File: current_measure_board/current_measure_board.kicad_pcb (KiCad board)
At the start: 6 copper layers, 76.2 x 76.2 mm, 43 parts, among them U1 LT6370HMS8-TRPBF, U2 LT1793AIS8-PBF, U3 LT1793AIS8-PBF, U4 LT1793AIS8-PBF

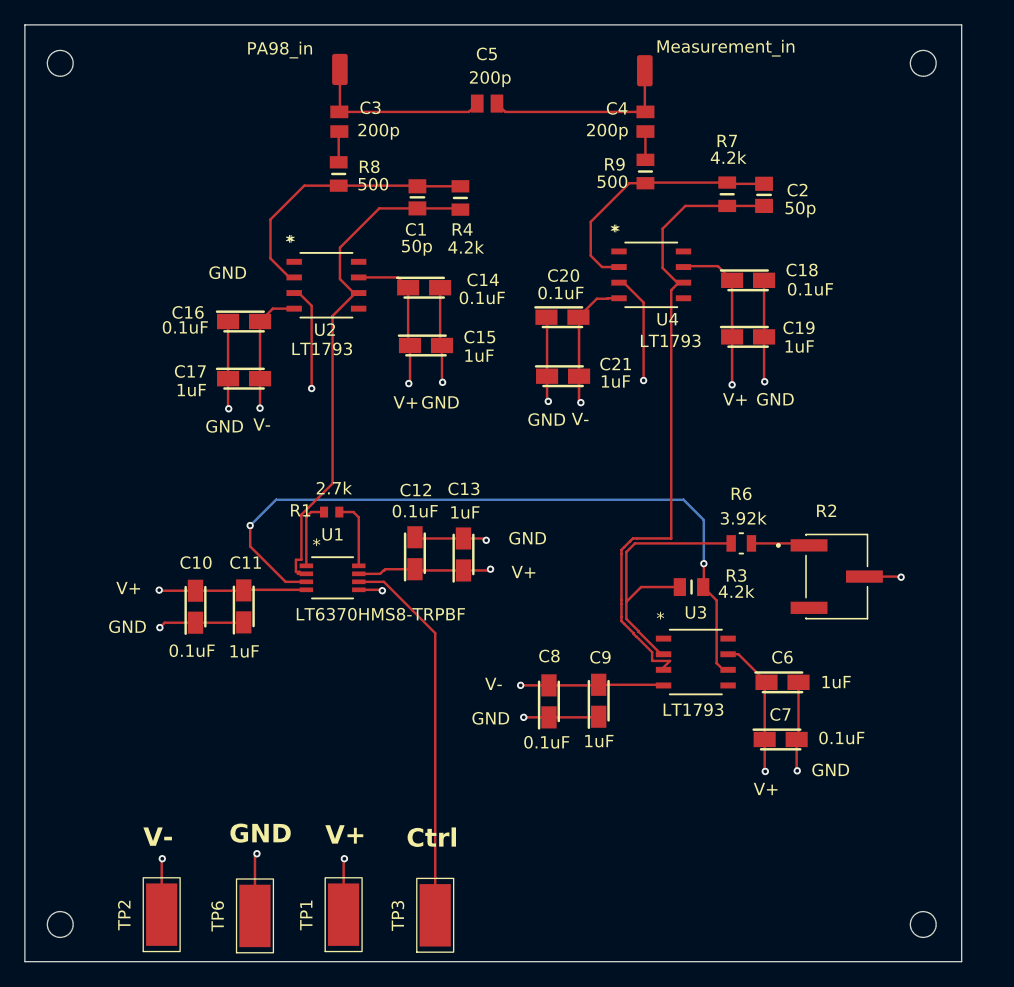
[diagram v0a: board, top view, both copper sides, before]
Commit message: current board update
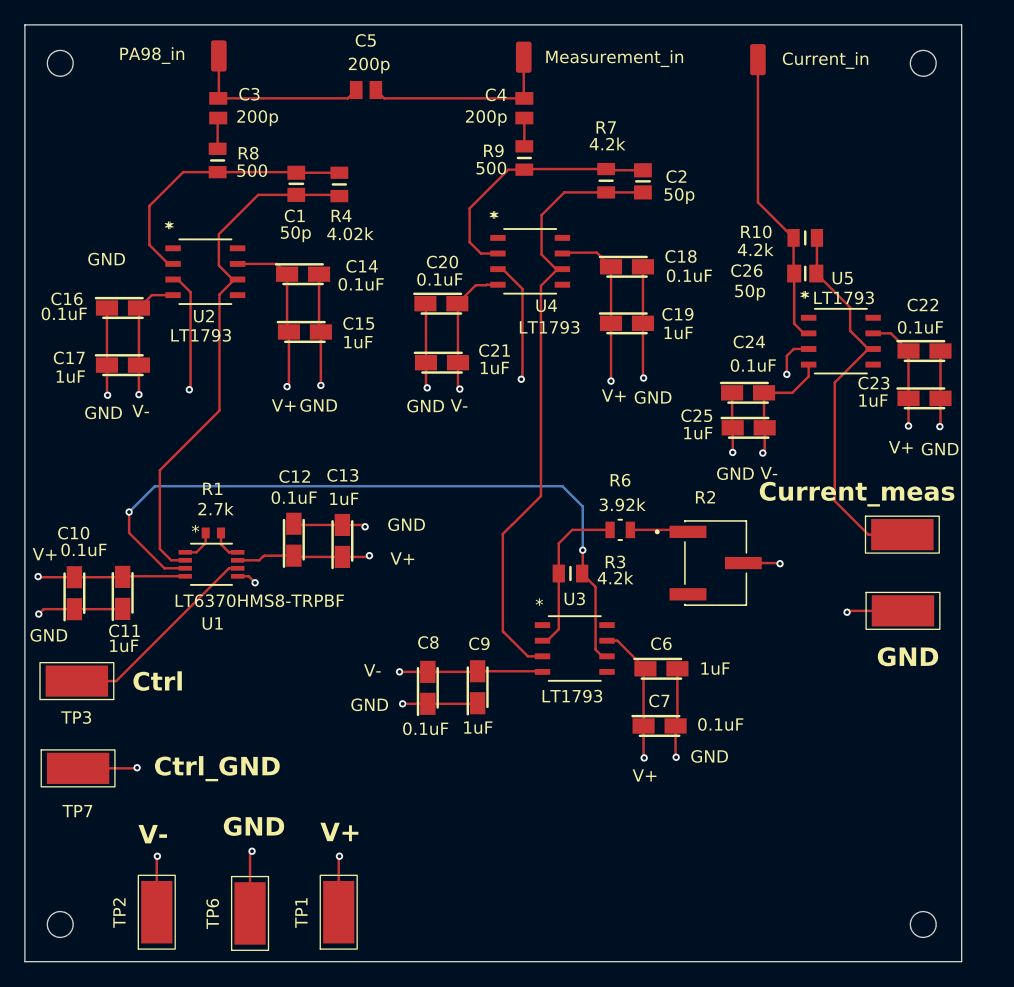
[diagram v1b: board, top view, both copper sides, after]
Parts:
- added C22: C1206C104K5RACTM, Custom_capacitors:CAPPM3216X180N(0.1uF 1206 0.1acc), F.Cu at (182.7, 84.2)
- added C23: TH3A105K035D6600, Custom_capacitors:CAPPM3216X180N(1uF 35V 1206 0.1err, F.Cu at (182.7, 88.1)
- added C24: C1206C104K5RACTM, Custom_capacitors:CAPPM3216X180N(0.1uF 1206 0.1acc), F.Cu at (168.3, 87.7)
- added C25: TH3A105K035D6600, Custom_capacitors:CAPPM3216X180N(1uF 35V 1206 0.1err, F.Cu at (168.4, 90.5)
- added C26: 50p, Custom_capacitors:CAPC2012X140N(50pF 1206 1 C0G 100V), F.Cu at (173.0, 78.0)
- added R10: 4.2k, Custom_resistors:RESC2012X55N(4.02k Ohm 0805 0.1err), F.Cu at (173.0, 75.0)
- added TP10: TestPoint, Custom_testpoint:PAD_EXT_0.635x2.54mm, F.Cu at (169.2, 60.5)
- added TP7: TestPoint, Custom_trimpot:PAD_EXT_2.54x5.08mm, F.Cu at (113.8, 120.7)
- added TP8: TestPoint, Custom_trimpot:PAD_EXT_2.54x5.08mm, F.Cu at (180.9, 101.7)
- added TP9: TestPoint, Custom_trimpot:PAD_EXT_2.54x5.08mm, F.Cu at (180.9, 107.9)
- added U5: LT1793AIS8-PBF, Custom_amplifiers:LT1793AIS_8_PBF, F.Cu at (175.9, 83.5)
- moved TP3 38.3 mm to (113.8, 108.6), turned to 180 degrees
- moved C21 9.91 mm to (143.4, 85.2)
- moved R6 9.91 mm to (157.9, 98.8)
- moved U4 9.91 mm to (150.6, 77.0)
- moved C10 9.91 mm to (113.5, 104.0)
- moved C11 9.91 mm to (117.5, 103.9)
- moved R8 9.91 mm to (125.2, 68.8)
- moved TP4 9.91 mm to (125.3, 60.2)
- moved U1 9.91 mm to (124.7, 101.6)
- moved U2 9.91 mm to (124.2, 77.8)
- moved C1 9.91 mm to (131.6, 70.7)
- moved C12 9.91 mm to (131.4, 99.6)
- moved C13 9.91 mm to (135.3, 99.7)
- moved C14 9.91 mm to (132.2, 78.0)
- moved C15 9.91 mm to (132.3, 82.7)
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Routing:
- net /Current_meas: track 0.00 -> 31.3 mm
- net GND: track 84.1 -> 112.2 mm, vias 13 -> 18
- net /Current_in: track 0.00 -> 24.2 mm
- net /Control_out: track 30.9 -> 16.9 mm
- net /Vplus: track 52.5 -> 64.3 mm, vias 5 -> 6
- net /Vminus: track 49.8 -> 59.9 mm, vias 5 -> 6
- net Net-(U3--INA): track 23.4 -> 13.5 mm
- net Net-(U1-RG+): track 5.70 -> 2.55 mm
- net Net-(U1-RG-): track 5.59 -> 2.80 mm
- net Net-(U3-+INA): track 53.4 -> 50.8 mm
- net Net-(U1-IN-): track 41.8 -> 42.5 mm
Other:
- board text added: "Ctrl_GND"
- board text added: "Current_in"
- board text added: "Current_meas"
